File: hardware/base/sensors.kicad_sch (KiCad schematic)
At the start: 11 parts, among them U2 FXOS8700CQR1, U3 MS5637-02BA03

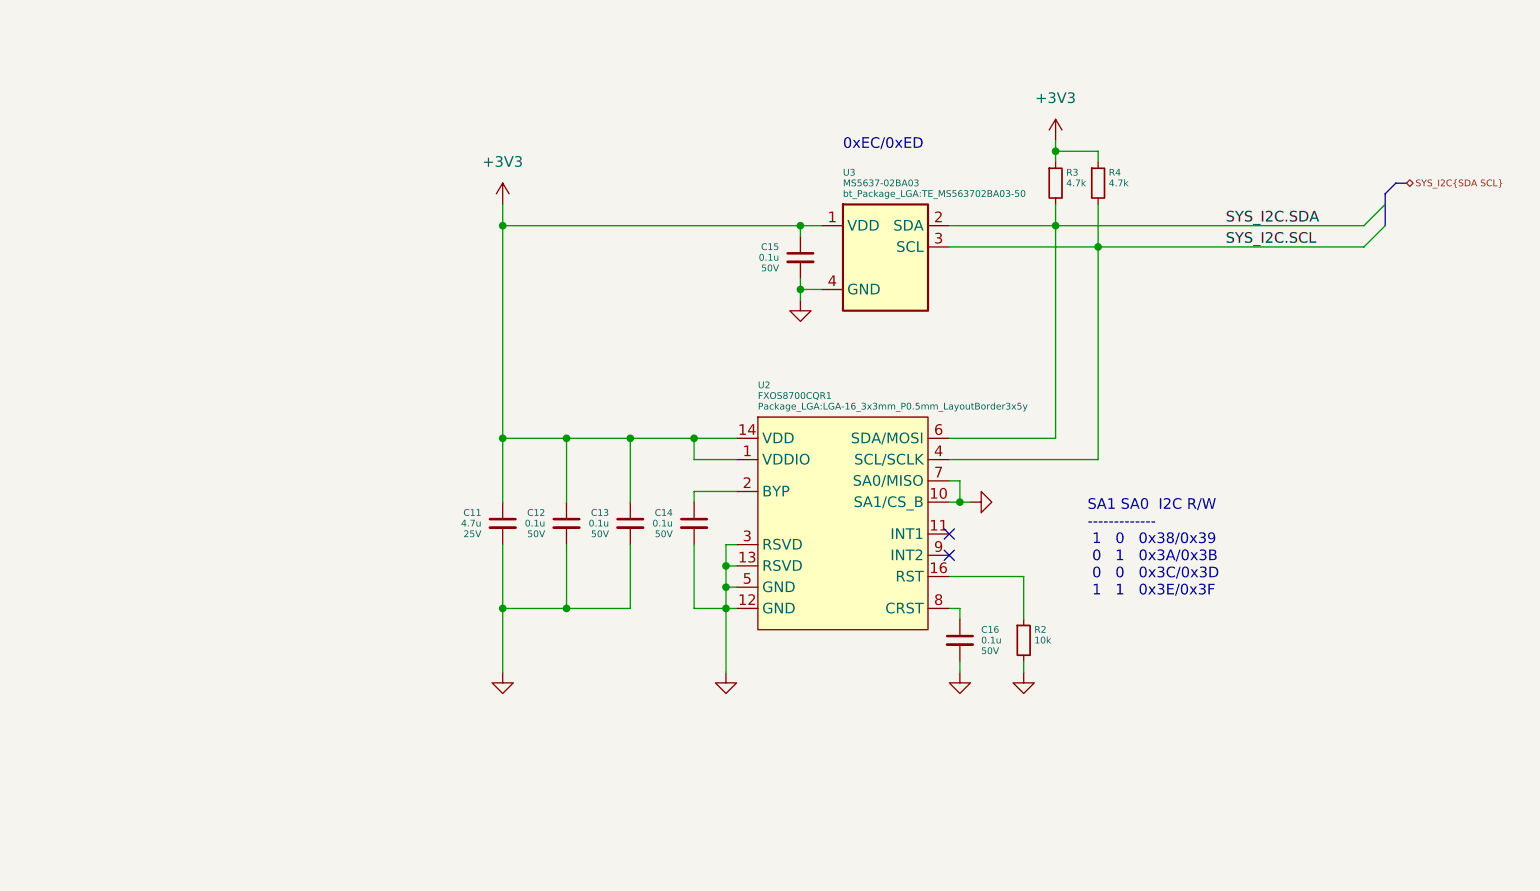
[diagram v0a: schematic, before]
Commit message: schematic complete unreviewed
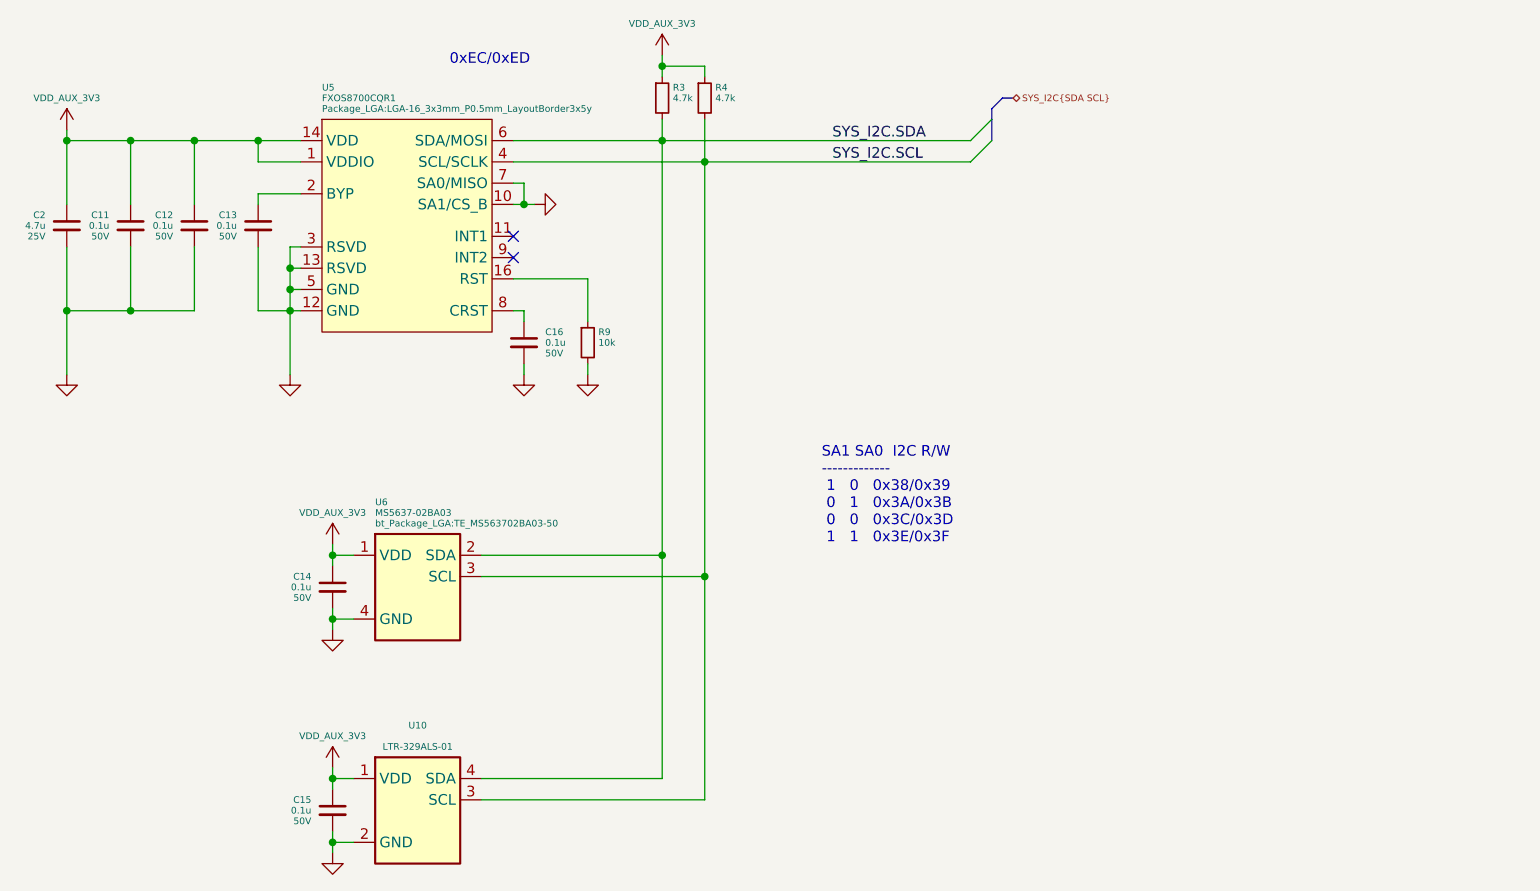
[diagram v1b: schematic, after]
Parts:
- removed R2: 10k, Resistor_SMD:R_0402_1005Metric, symbol Device:R_Small
- removed U2: FXOS8700CQR1, Package_LGA:LGA-16_3x3mm_P0.5mm_LayoutBorder3x5y, symbol bt_Sensor_Motion:FXOS8700CQR1
- removed U3: MS5637-02BA03, bt_Package_LGA:TE_MS563702BA03-50, symbol bt_Sensor_Environmental:MS5637-02BA03
- added C2: 4.7u, Capacitor_SMD:C_0603_1608Metric, symbol Device:C_Small
- added R9: 10k, Resistor_SMD:R_0402_1005Metric, symbol Device:R_Small
- added U10: LTR-329ALS-01, Package_LGA:VLGA-4_2x2.5mm_P1.65mm, symbol bt_Sensor_Environmental:LTR-329ALS-01
- added U5: FXOS8700CQR1, Package_LGA:LGA-16_3x3mm_P0.5mm_LayoutBorder3x5y, symbol bt_Sensor_Motion:FXOS8700CQR1
- added U6: MS5637-02BA03, bt_Package_LGA:TE_MS563702BA03-50, symbol bt_Sensor_Environmental:MS5637-02BA03
- C11: value 4.7u -> 0.1u; footprint Capacitor_SMD:C_0603_1608Metric -> Capacitor_SMD:C_0402_1005Metric; Voltage 25V -> 50V
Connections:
- net GND: now also C2.2, R9.2, U10.2 (GND), U5.10 (SA1/CS_B), U5.12 (GND), U5.13 (RSVD), U5.3 (RSVD), U5.5 (GND), U5.7 (SA0/MISO), U6.4 (GND)
- net SYS_I2C.SCL: now also U10.3 (SCL), U5.4 (SCL/SCLK), U6.3 (SCL)
- net SYS_I2C.SDA: now also U10.4 (SDA), U5.6 (SDA/MOSI), U6.2 (SDA)
- net VDD_AUX_3V3: now reaches C14.1
- net VDD_AUX_3V3: now also C11.1, C12.1, C15.1, R3.1, R4.1, C2.1, U10.1 (VDD), U5.1 (VDDIO), U5.14 (VDD), U6.1 (VDD)
- net at C16.1: now also U5.8 (CRST)
- removed net +3V3: C11.1, C12.1, C13.1, C15.1, R3.1, R4.1
- new net: R9.1, U5.16 (RST)
- new net: C13.1, U5.2 (BYP)
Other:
- moved on the sheet: R3, R4
